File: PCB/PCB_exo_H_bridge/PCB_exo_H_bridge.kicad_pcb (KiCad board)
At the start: 4 copper layers, 30 x 30 mm, 15 parts, among them J201 USB_C_Receptacle_USB2.0, U201 STM32G4A1REIx, U202 USBLC6-2SC6

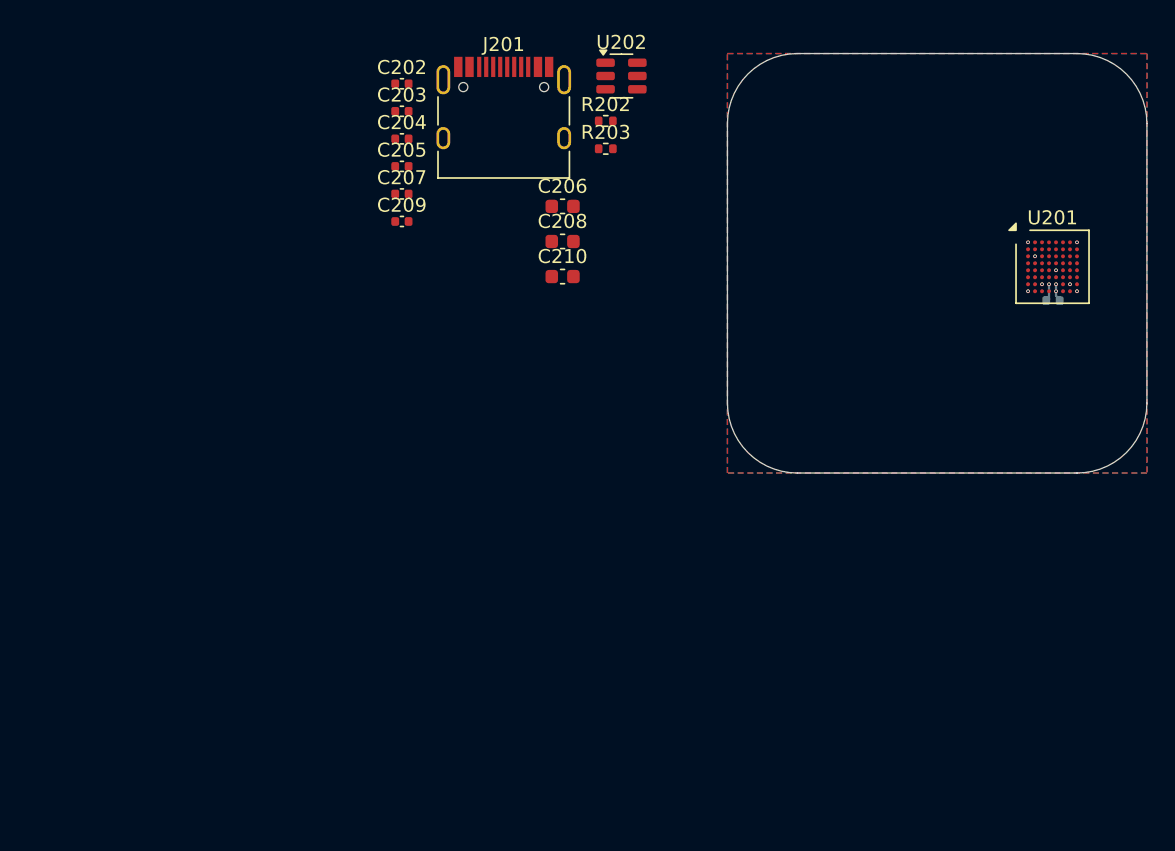
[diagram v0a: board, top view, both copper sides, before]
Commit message: exo done
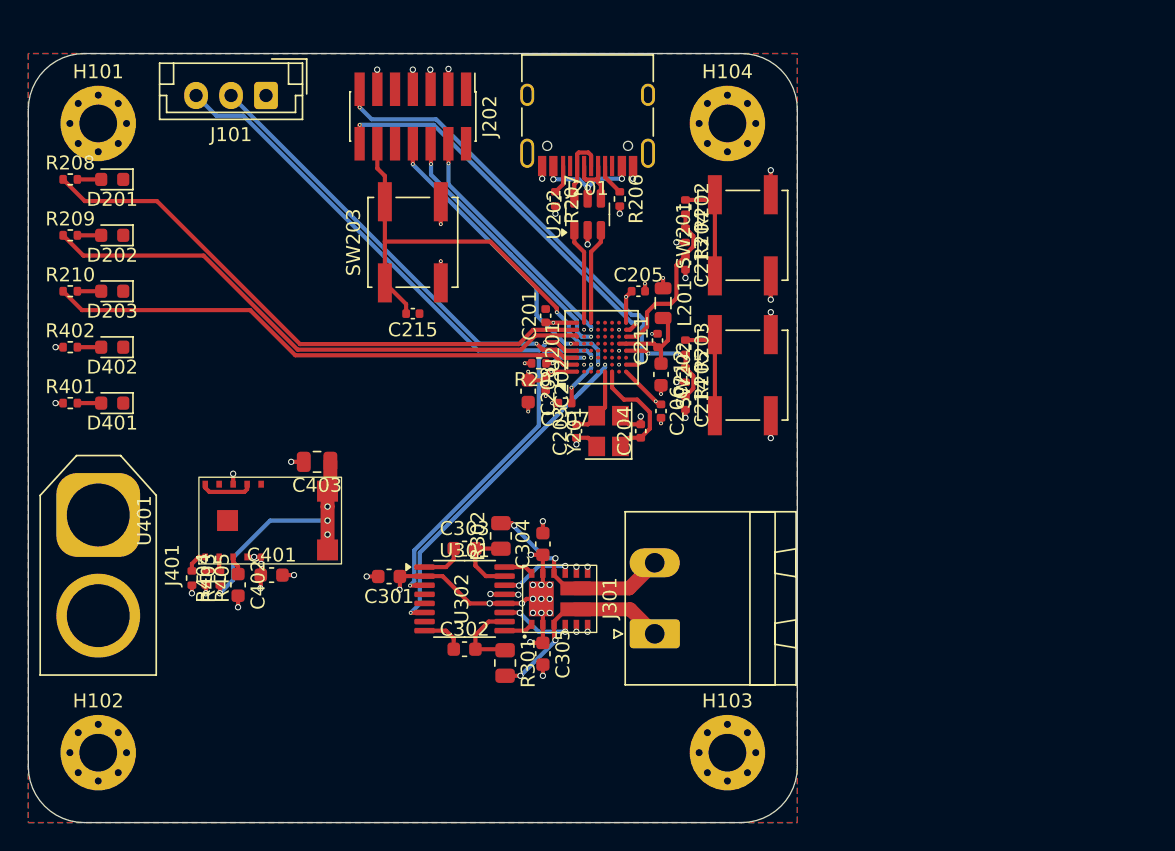
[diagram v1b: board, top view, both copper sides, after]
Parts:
- removed C209: 100n, Capacitor_SMD:C_0402_1005Metric
- removed C210: 1u, Capacitor_SMD:C_0603_1608Metric
- added C211: 100n, Capacitor_SMD:C_0402_1005Metric, F.Cu at (90.0, 65.5)
- added C212: 1u, Capacitor_SMD:C_0603_1608Metric, F.Cu at (90.2, 68.0)
- added C213: 100n, Capacitor_SMD:C_0402_1005Metric, F.Cu at (92.0, 60.0)
- added C214: 100n, Capacitor_SMD:C_0402_1005Metric, F.Cu at (92.0, 70.0)
- added C215: 100n, Capacitor_SMD:C_0402_1005Metric, F.Cu at (72.5, 63.6)
- added C301: 2u2, Capacitor_SMD:C_0603_1608Metric, F.Cu at (70.8, 82.4)
- added C302: 1u, Capacitor_SMD:C_0603_1608Metric, F.Cu at (76.2, 87.6)
- added C303: 1u, Capacitor_SMD:C_0603_1608Metric, F.Cu at (76.2, 80.4)
- added C304: 10u, Capacitor_SMD:C_0603_1608Metric, F.Cu at (81.8, 80.1)
- added C305: 10u, Capacitor_SMD:C_0603_1608Metric, F.Cu at (81.8, 87.9)
- added C401: 10u, Capacitor_SMD:C_0603_1608Metric, F.Cu at (62.4, 82.3)
- added C402: 1u, Capacitor_SMD:C_0603_1608Metric, F.Cu at (60.0, 83.0)
- added C403: 47u, Capacitor_SMD:C_0805_2012Metric, F.Cu at (65.7, 74.2)
- added D201: LED Red, LED_SMD:LED_0603_1608Metric, F.Cu at (51.0, 54.0)
- added D202: LED Amber, LED_SMD:LED_0603_1608Metric, F.Cu at (51.0, 58.0)
- added D203: LED Yellow, LED_SMD:LED_0603_1608Metric, F.Cu at (51.0, 62.0)
- added D401: LED_Blue, LED_SMD:LED_0603_1608Metric, F.Cu at (51.0, 70.0)
- added D402: LED_Green, LED_SMD:LED_0603_1608Metric, F.Cu at (51.0, 66.0)
- added H101: MountingHole_Pad, MountingHole:MountingHole_2.7mm_M2.5_Pad_Via, F.Cu at (50.0, 50.0)
- added H102: MountingHole_Pad, MountingHole:MountingHole_2.7mm_M2.5_Pad_Via, F.Cu at (50.0, 95.0)
- added H103: MountingHole_Pad, MountingHole:MountingHole_2.7mm_M2.5_Pad_Via, F.Cu at (95.0, 95.0)
- added H104: MountingHole_Pad, MountingHole:MountingHole_2.7mm_M2.5_Pad_Via, F.Cu at (95.0, 50.0)
- added J101: Conn_01x03, Connector_JST:JST_EH_B3B-EH-A_1x03_P2.50mm_Vertical, F.Cu at (62.0, 48.0)
- added J202: Conn_ST_STDC14, Connector_PinHeader_1.27mm:PinHeader_2x07_P1.27mm_Vertical_SMD, F.Cu at (72.5, 49.5)
- added J301: Conn_01x02, Connector_Phoenix_MSTB:PhoenixContact_MSTBA_2,5_2-G-5,08_1x02_P5.08mm_Horizontal, F.Cu at (89.8, 86.5)
- added J401: Conn_01x02, Connector_AMASS:AMASS_XT60-F_1x02_P7.20mm_Vertical, F.Cu at (50.0, 78.0)
- added L201: 39n, Inductor_SMD:L_0805_2012Metric, F.Cu at (90.4, 62.9)
- added R201: 10k, Resistor_SMD:R_0402_1005Metric, F.Cu at (81.5, 67.2)
- added R204: 10k, Resistor_SMD:R_0402_1005Metric, F.Cu at (92.0, 58.0)
- added R205: 10k, Resistor_SMD:R_0402_1005Metric, F.Cu at (92.0, 68.0)
- added R206: 5.1k, Resistor_SMD:R_0402_1005Metric, F.Cu at (87.3, 55.4)
- added R207: 5.1k, Resistor_SMD:R_0402_1005Metric, F.Cu at (82.7, 55.4)
- added R208: 1k7, Resistor_SMD:R_0402_1005Metric, F.Cu at (48.0, 54.0)
- added R209: 1k7, Resistor_SMD:R_0402_1005Metric, F.Cu at (48.0, 58.0)
- added R210: 1k7, Resistor_SMD:R_0402_1005Metric, F.Cu at (48.0, 62.0)
- added R301: 3, Resistor_SMD:R_0805_2012Metric, F.Cu at (79.1, 88.6)
- added R302: 3, Resistor_SMD:R_0805_2012Metric, F.Cu at (78.8, 79.5)
- added R401: 12k2, Resistor_SMD:R_0402_1005Metric, F.Cu at (48.0, 70.0)
- added R402: 1k, Resistor_SMD:R_0402_1005Metric, F.Cu at (48.0, 66.0)
- added R403: 5k6, Resistor_SMD:R_0402_1005Metric, F.Cu at (56.7, 82.5)
- added R404: 287k, Resistor_SMD:R_0402_1005Metric, F.Cu at (58.7, 82.5)
- added R405: 100k, Resistor_SMD:R_0402_1005Metric, F.Cu at (57.7, 82.5)
- added SW201: SW_Push, Button_Switch_SMD:SW_Push_1P1T_NO_CK_KSC6xxJ, F.Cu at (96.1, 58.0)
- added SW202: SW_Push, Button_Switch_SMD:SW_Push_1P1T_NO_CK_KSC6xxJ, F.Cu at (96.1, 68.0)
- added SW203: SW_Push, Button_Switch_SMD:SW_Push_1P1T_NO_CK_KSC6xxJ, F.Cu at (72.5, 58.5)
- added U301: IC4606-2YTS-TR, Package_SO:TSSOP-16_4.4x5mm_P0.65mm, F.Cu at (76.2, 84.0)
- added U302: FDMQ86530L, Maker_librairy:FDMQ86530L, F.Cu at (83.0, 84.0)
- added U401: 171013801, Maker_librairy:171013801, F.Cu at (62.3, 78.4)
- added Y201: Crystal_GND24, Crystal:Crystal_SMD_3225-4Pin_3.2x2.5mm, F.Cu at (86.5, 72.0)
- C201: moved to F.Cu
- C203, C204: value 100n -> 12p
- C206: value 10u -> 100n; footprint Capacitor_SMD:C_0603_1608Metric -> Capacitor_SMD:C_0402_1005Metric
- C208: value 1u -> 10u
- R202, R203: value 5.1k -> 10k
- moved C201 36.3 mm to (82.0, 63.8), turned to 90 degrees
- moved U201 32.8 mm to (86.0, 66.0), turned to 90 degrees
- moved C204 27.0 mm to (88.8, 72.0), turned to 90 degrees
- moved C203 26.1 mm to (84.2, 72.0), turned to 90 degrees
- moved C202 23.8 mm to (82.0, 68.6), turned to -90 degrees
- moved C205 19.1 mm to (88.6, 62.0)
- moved C207 19.0 mm to (83.4, 70.0), turned to 180 degrees
- moved C206 16.2 mm to (90.2, 70.6), turned to -90 degrees
- moved R203 15.3 mm to (92.0, 66.0), turned to -90 degrees
- moved C208 11.0 mm to (80.8, 69.2), turned to -90 degrees
- moved U202 10.2 mm to (85.0, 56.5), turned to 90 degrees
- moved R202 8.39 mm to (92.0, 56.0), turned to -90 degrees
- moved J201 6.08 mm to (85.0, 49.0), turned to 180 degrees
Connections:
- C203 pad 1: +3.3V -> GND
- C203 pad 2: GND -> Net-(U201-PF0)
- C204 pad 1: +3.3V -> Net-(U201-PF1)
- C207 pad 1: +3.3VA -> +3.3V
- C208 pad 1: +3.3VA -> +3.3V
- R202 pad 1: Net-(J201-CC1) -> Net-(R202-Pad1)
- R202 pad 2: Net-(R202-Pad2) -> /STM32G4A1REI6_ref_design/USR_BTN_1
- R203 pad 1: Net-(J201-CC2) -> Net-(R203-Pad1)
- R203 pad 2: Net-(R202-Pad2) -> /STM32G4A1REI6_ref_design/USR_BTN_2
- U201 pad A2: unconnected-(U201-PB9-PadA2) -> /STM32G4A1REI6_ref_design/USR_LED_3
- U201 pad A6: /STM32G4A1REI6_ref_design/USR_BTN_1 -> /STM32G4A1REI6_ref_design/USR_LED_2
- U201 pad A7: /STM32G4A1REI6_ref_design/USR_BTN_2 -> /STM32G4A1REI6_ref_design/USR_LED_1
- U201 pad B1: /STM32G4A1REI6_ref_design/PWM_CH1N -> unconnected-(U201-PC13-PadB1)
- U201 pad C3: /STM32G4A1REI6_ref_design/PWM_CH2 -> /IC4606-2_FDMQ86530L_Motor_driver/PWM_B
- U201 pad E2: /STM32G4A1REI6_ref_design/PWM_CH1 -> /IC4606-2_FDMQ86530L_Motor_driver/PWM_A
- U201 pad E5: /STM32G4A1REI6_ref_design/PWM_CH2N -> unconnected-(U201-PB0-PadE5)
- U201 pad E8: /STM32G4A1REI6_ref_design/USR_LED_1 -> unconnected-(U201-PC6-PadE8)
- U201 pad F8: /STM32G4A1REI6_ref_design/USR_LED_2 -> unconnected-(U201-PB14-PadF8)
- U201 pad G5: +3.3V -> +3.3VA
- U201 pad G8: /STM32G4A1REI6_ref_design/USR_LED_3 -> unconnected-(U201-PB12-PadG8)
- U201 pad H4: unconnected-(U201-PB2-PadH4) -> /STM32G4A1REI6_ref_design/USR_BTN_2
- U201 pad H5: +3.3V -> +3.3VA
- U201 pad H6: unconnected-(U201-PB10-PadH6) -> /STM32G4A1REI6_ref_design/USR_BTN_1
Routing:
- net /STM32G4A1REI6_ref_design/USR_LED_1: track 0.00 -> 42.1 mm
- net VCC: track 0.00 -> 41.5 mm, vias 0 -> 18
- net /STM32G4A1REI6_ref_design/USR_LED_2: track 0.00 -> 40.6 mm
- net /STM32G4A1REI6_ref_design/USR_LED_3: track 0.00 -> 38.9 mm
- net GND: track 1.23 -> 38.7 mm, vias 2 -> 46
- net +3.3V: track 1.34 -> 37.7 mm, vias 7 -> 16
- net /STM32G4A1REI6_ref_design/UART_TX: track 0.00 -> 35.4 mm, vias 0 -> 1
- net /STM32G4A1REI6_ref_design/NRST: track 0.00 -> 33.0 mm, vias 0 -> 2
- net /STM32G4A1REI6_ref_design/UART_RX: track 0.00 -> 32.5 mm, vias 0 -> 1
- net /STM32G4A1REI6_ref_design/VCP_RX: track 0.00 -> 32.1 mm, vias 0 -> 2
- net /IC4606-2_FDMQ86530L_Motor_driver/PWM_A: track 0.00 -> 29.8 mm, vias 0 -> 2
- net /STM32G4A1REI6_ref_design/VCP_TX: track 0.00 -> 28.1 mm, vias 0 -> 2
- net /IC4606-2_FDMQ86530L_Motor_driver/PWM_B: track 0.00 -> 25.4 mm, vias 0 -> 2
- net /STM32G4A1REI6_ref_design/SWO: track 0.00 -> 19.7 mm, vias 0 -> 2
- net /STM32G4A1REI6_ref_design/SWCLK: track 0.00 -> 18.9 mm, vias 0 -> 2
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- added copper zone on In2.Cu, net VCC
- removed copper zone on In2.Cu, net +5V
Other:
- board size 30 x 30 mm -> 55 x 55 mm
